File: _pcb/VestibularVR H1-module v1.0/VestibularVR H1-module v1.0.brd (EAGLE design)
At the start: 57.1 x 58.2 mm, 46 parts, among them IC1 FT232RL, IC2 74LVC1G07DBV, IC4 74LVC1G07DBV, IC5 74LVC1G07DBV, IC6 74LVC1G07DBV, IC9 USBLC6-2SC6, J1 reward_valve_1, J2 reward_valve_2, J3 lick_port_1, J4 lick_port_2, J5 Optical_flow_1, J6 Optical_flow_2, J7 Camera_trigger_1, J8 Camera_trigger_2

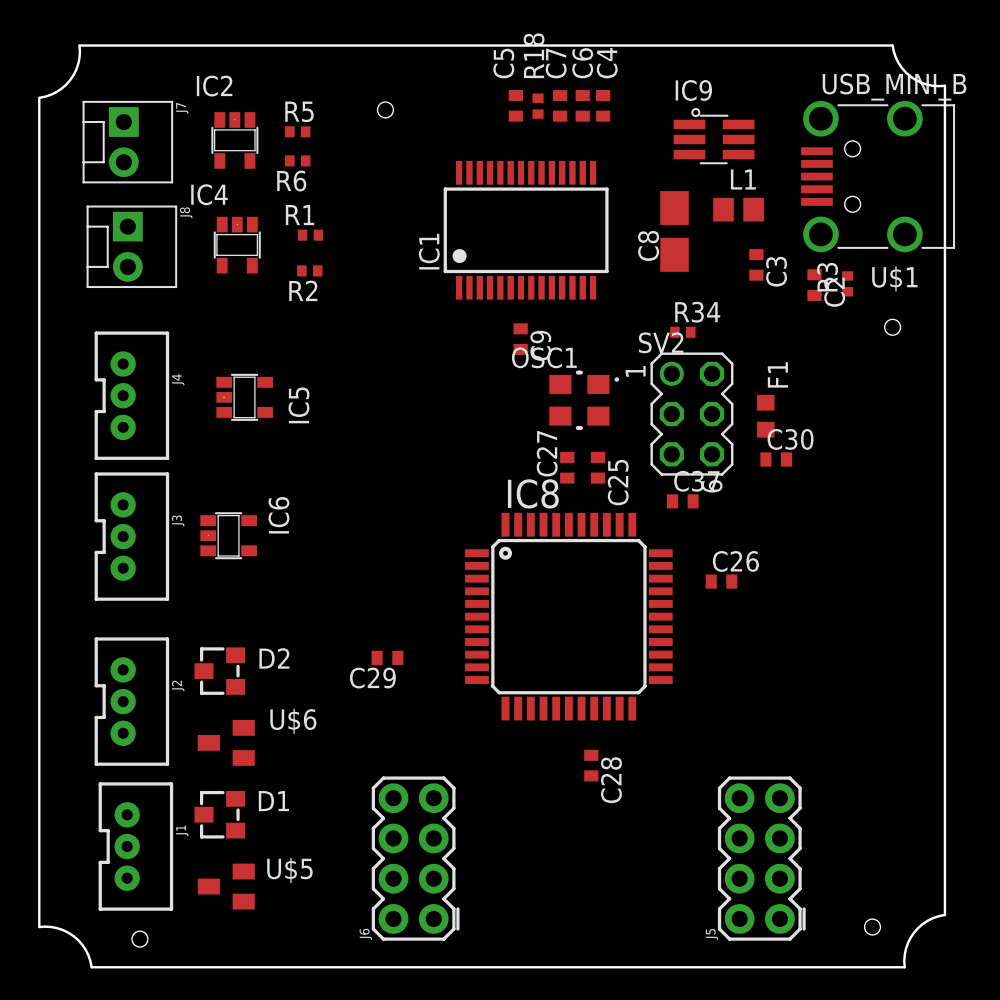
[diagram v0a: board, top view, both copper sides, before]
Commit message: proceeding design VestibularVR H1
- Eagle version changed back to v.8.3.1
- proceeding design VestibularVR H1-module v1.0
- added Lick Sensor module v1.0
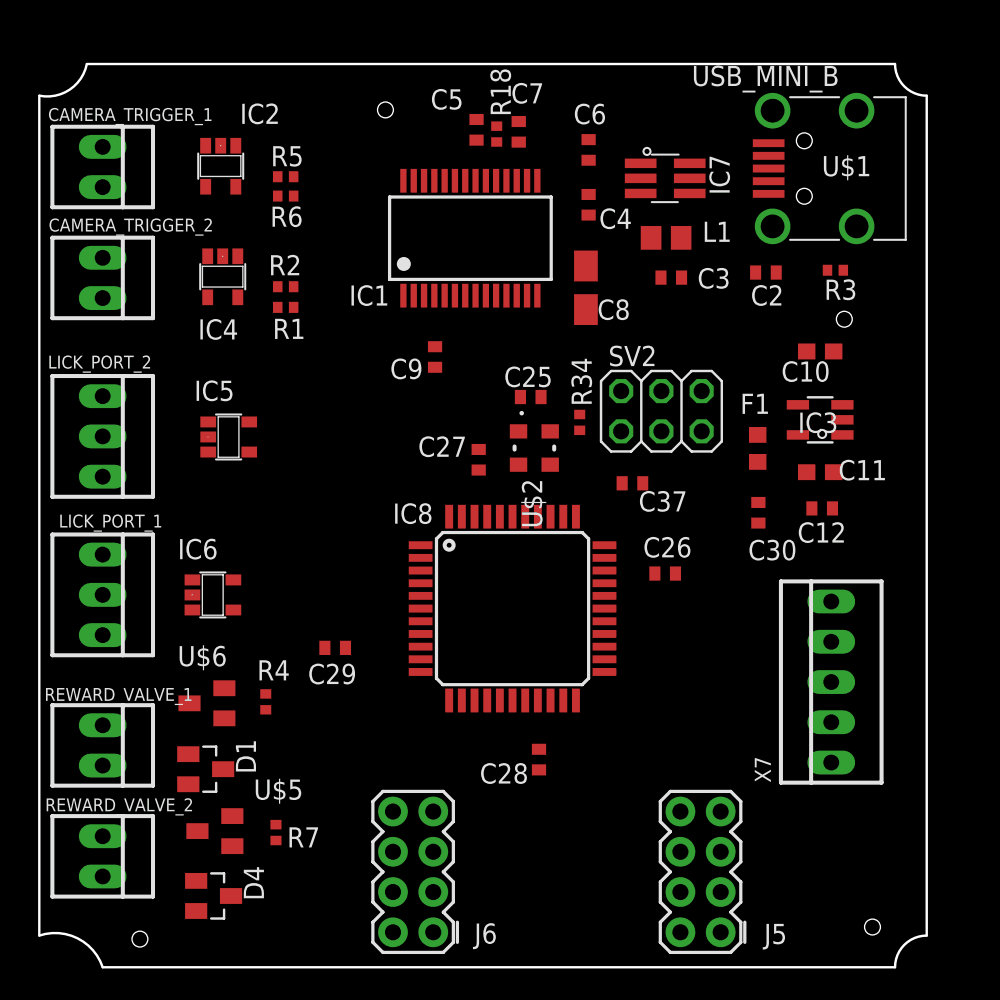
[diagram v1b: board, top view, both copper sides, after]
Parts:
- removed D2: BZX84CSMD, diode:TO236
- removed IC9: USBLC6-2SC6, VestibularVR H1-module v1.0:SOT23-6L
- removed J1: reward_valve_1, SparkFun-Connectors:JST-3-PTH-VERT
- removed J2: reward_valve_2, SparkFun-Connectors:JST-3-PTH-VERT
- removed J3: lick_port_1, SparkFun-Connectors:JST-3-PTH-VERT
- removed J4: lick_port_2, SparkFun-Connectors:JST-3-PTH-VERT
- removed J7: Camera_trigger_1, SparkFun-Connectors:MOLEX-1X2
- removed J8: Camera_trigger_2, SparkFun-Connectors:MOLEX-1X2
- removed OSC1: OSCILLATOR, harp camera controller:OSCILLATOR_3.2X2.5
- added C10, C11: 4.7uF, rcl:C0603
- added C12: 100nF, rcl:C0402
- added CAMERA_TRIGGER_1, CAMERA_TRIGGER_2, REWARD_VALVE_1, REWARD_VALVE_2: 22-23-2021, con-molex:22-23-2021
- added D4: BAT54, diode:SOT23
- added IC3: TLV70033DDCR, VestibularVR H1-module v1.0:TSOT23-5
- added IC7: USBLC6-2SC6, VestibularVR H1-module v1.0:SOT23-6L
- added LICK_PORT_1, LICK_PORT_2: 22-23-2031, con-molex:22-23-2031
- added R4, R7: 10k, rcl:R0402
- added U$2: OSCILLATOR, VestibularVR H1-module v1.0:OSCILLATOR_3.2X2.5
- added X7: 22-23-2051, con-molex:22-23-2051
- C8: device rcl:A/3216-18W -> rcl:A/3216-18R
- D1: value BZX84CSMD -> BAT54; device diode:TO236 -> diode:SOT23
- F1: device harp camera controller:R0603 -> VestibularVR H1-module v1.0:R0603
- IC8: value (none) -> ATXMEGA32A4U
- SV2: value (none) -> PINHD-2X3; device con-lstb:MA03-2 -> Connector:2X03
- moved R34 8.64 mm to (34.1, 34.4), turned to 90 degrees
- moved C8 6.62 mm to (34.5, 42.9)
- moved C4 6.31 mm to (34.7, 48.1), turned to 270 degrees
- moved C25 6.16 mm to (31.0, 36.0), turned to 180 degrees
- moved C27 5.61 mm to (27.7, 32.0)
- moved C9 5.52 mm to (25.0, 38.5)
- moved C3 5.43 mm to (39.9, 43.5), turned to 180 degrees
- moved L1 4.91 mm to (39.6, 46.0)
- moved R1 4.82 mm to (15.5, 41.6)
- moved R5 4.13 mm to (15.5, 48.7)
- moved IC6 3.87 mm to (10.9, 23.5)
- moved J5 3.83 mm to (41.7, 6.02)
- moved IC8 3.59 mm to (29.9, 22.6)
- moved C26 3.59 mm to (39.5, 24.8)
- moved U$5 3.57 mm to (11.1, 8.59)
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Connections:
- removed net N$15: C5.1, C8.+, IC1.20, L1.1
- removed net U_HARP_H1_BOARD_RX: IC8.22
- removed net U_HARP_H1_BOARD_TX: IC8.23
- removed net VDD: C25.1, C26.1, C27.1, C28.1, C29.1, C30.1, F1.1, IC8.19, IC8.31, IC8.39, IC8.9, OSC1.P$4, R34.2, SV2.6
- new net +12V: X7.5
- new net +3V3_U: C25.1, C26.1, C27.1, C28.1, C29.1, C30.1, F1.1, IC8.19, IC8.31, IC8.39, IC8.9, R34.2, SV2.6, U$2.P$4
- new net HARP_H1_BOARD_RX: IC8.22, X7.3
- new net HARP_H1_BOARD_TX: IC8.23, X7.4
- new net HARP_H1_CLOCK_IN: IC8.12, X7.2
- new net N$7: D4.3, REWARD_VALVE_2.2
- new net N$8: D1.3, REWARD_VALVE_1.2
- net +3V3: now also C11.1, C12.1, IC3.5, IC5.5, IC6.5, LICK_PORT_1.3, LICK_PORT_2.3; no longer J3.3, J4.3
- net +5V: now also C10.1, C5.1, C8.+, IC1.20, IC3.1, IC3.3, L1.1; no longer D1.C, D2.C, J1.3, J2.3
- net GND: now also C10.2, C11.2, C12.2, CAMERA_TRIGGER_1.1, CAMERA_TRIGGER_2.1, IC3.2, IC7.P$2, LICK_PORT_1.1, LICK_PORT_2.1, R4.1, R7.1, U$2.P$2, X7.1; no longer IC9.P$2, J3.1, J4.1, J7.1, J8.1, OSC1.P$2
- net LICK_PORT_1: now also LICK_PORT_1.2; no longer J3.2
- net LICK_PORT_2: now also LICK_PORT_2.2; no longer J4.2
- net N$16: now also CAMERA_TRIGGER_1.2; no longer J7.2
- net N$2: now also IC7.P$4; no longer IC9.P$6
- net N$3: now also IC7.P$6; no longer IC9.P$4
- net N$4: now also CAMERA_TRIGGER_2.2; no longer J8.2
- net N$6: now also D4.1, REWARD_VALVE_2.1; no longer D1.A, J2.1
- net N$9: now also D1.1, REWARD_VALVE_1.1; no longer D2.A, J1.1
- net OSC2: now also U$2.P$3; no longer OSC1.P$3
- net USBDM: now also IC7.P$1; no longer IC9.P$3
- net USBDP: now also IC7.P$3; no longer IC9.P$1
- net USB_POWER: now also IC7.P$5; no longer IC9.P$5
- net U_CAM2_TRIGGER: now also IC8.20; no longer IC8.5
- net U_OPTICAL_FLOW_1_INT: no longer IC8.20
- net U_OPTICAL_FLOW_2_INT: no longer IC8.21
- net U_REWARD_VALVE_1: now also R4.2
- net U_REWARD_VALVE_2: now also R7.2
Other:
- board size 57.1 x 58.2 mm -> 56 x 57 mm
